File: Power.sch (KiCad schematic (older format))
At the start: 80 parts, among them J3 USB, J4 OTG, Q1 DTA114YKA, SW1 PWRON, SW2 RST, U1 AllWinner-S3(FBGA-234), U3 AXP209(QFN-48), U4 SY8089AAAC, U5 SY6280AAC

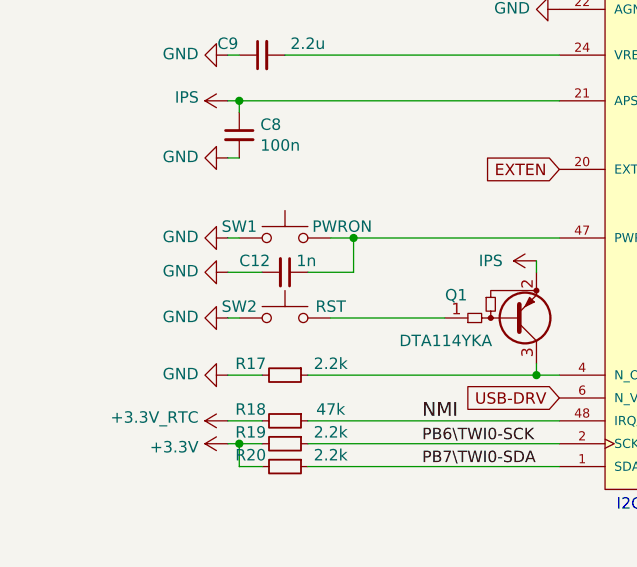
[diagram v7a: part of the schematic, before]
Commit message: update
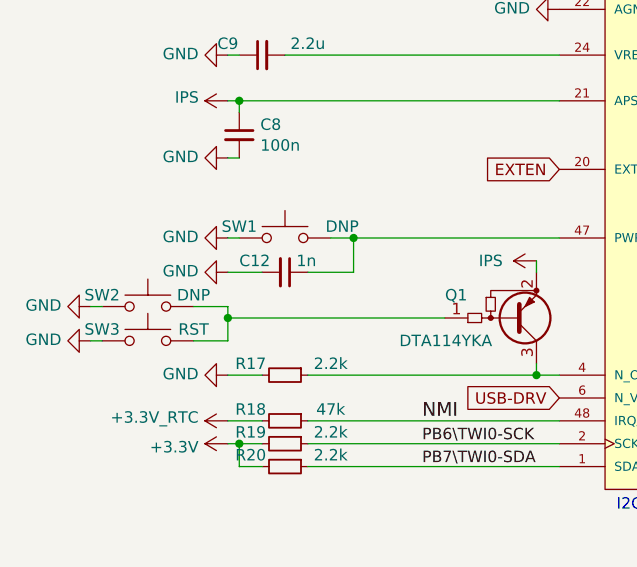
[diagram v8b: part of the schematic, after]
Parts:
- added SW3: RST, otter:SW_SPST_PTS810, symbol Switch:SW_Push
- SW1: value PWRON -> DNP; footprint Button_Switch_SMD:SW_SPST_PTS810 -> otter:SW_SPST_PTS810
- SW2: value RST -> DNP; footprint Button_Switch_SMD:SW_SPST_PTS810 -> otter:SW_SPST_PTS810
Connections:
- net GND: now also SW3.1
- net at Q1.1 (B), SW2.2: now also SW3.2
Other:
- moved on the sheet: SW2
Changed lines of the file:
@@
 L Switch:SW_Push SW2
 U 1 1 6637168B
-P 2050 5300
-F 0 "SW2" H 1850 5350 50  0000 C CNN
-F 1 "RST" H 2250 5350 50  0000 C CNN
-F 2 "Button_Switch_SMD:SW_SPST_PTS810" H 2050 5500 50  0001 C CNN
-F 3 "~" H 2050 5500 50  0001 C CNN
-	1    2050 5300
+P 1450 5250
+F 0 "SW2" H 1250 5300 50  0000 C CNN
+F 1 "DNP" H 1650 5300 50  0000 C CNN
+F 2 "otter:SW_SPST_PTS810" H 1450 5450 50  0001 C CNN
+F 3 "~" H 1450 5450 50  0001 C CNN
+	1    1450 5250
 	1    0    0    -1
 $EndComp
@@
 L S3-OLinuXino_Rev_A:GND #PWR?
 U 1 1 663B8CCA
-P 1800 5300
+P 1200 5250
 AR Path="/5D8A1FAC/663B8CCA" Ref="#PWR?"  Part="1"
 AR Path="/663B8CCA" Ref="#PWR?"  Part="1"
 AR Path="/602ACDF9/663B8CCA" Ref="#PWR0165"  Part="1"
-F 0 "#PWR0165" H 1800 5050 50  0001 C CNN
-F 1 "GND" V 1805 5172 50  0000 R CNN
-F 2 "" H 1800 5300 60  0000 C CNN
-F 3 "" H 1800 5300 60  0000 C CNN
-	1    1800 5300
+F 0 "#PWR0165" H 1200 5000 50  0001 C CNN
+F 1 "GND" V 1205 5122 50  0000 R CNN
+F 2 "" H 1200 5250 60  0000 C CNN
+F 3 "" H 1200 5250 60  0000 C CNN
+	1    1200 5250
 	0    1    -1   0
 $EndComp
 Wire Wire Line
-	1850 5300 1800 5300
+	1250 5250 1200 5250
 $Comp
 L Device:C_Small C?
@@
 P 2050 4950
 F 0 "SW1" H 1850 5000 50  0000 C CNN
-F 1 "PWRON" H 2300 5000 50  0000 C CNN
-F 2 "Button_Switch_SMD:SW_SPST_PTS810" H 2050 5150 50  0001 C CNN
+F 1 "DNP" H 2300 5000 50  0000 C CNN
+F 2 "otter:SW_SPST_PTS810" H 2050 5150 50  0001 C CNN
 F 3 "~" H 2050 5150 50  0001 C CNN
 	1    2050 4950
@@
 $EndComp
 Wire Wire Line
-	2250 5300 2750 5300
-Wire Wire Line
 	2150 5100 2350 5100
 Wire Wire Line
@@
 Wire Wire Line
 	10850 4800 11450 4800
+$Comp
+L Switch:SW_Push SW3
+U 1 1 601100C1
+P 1450 5400
+F 0 "SW3" H 1250 5450 50  0000 C CNN
+F 1 "RST" H 1650 5450 50  0000 C CNN
+F 2 "otter:SW_SPST_PTS810" H 1450 5600 50  0001 C CNN
+F 3 "~" H 1450 5600 50  0001 C CNN
+	1    1450 5400
+	1    0    0    -1
+$EndComp
+$Comp
+L S3-OLinuXino_Rev_A:GND #PWR?
+U 1 1 60166E26
+P 1200 5400
+AR Path="/5D8A1FAC/60166E26" Ref="#PWR?"  Part="1"
+AR Path="/60166E26" Ref="#PWR?"  Part="1"
+AR Path="/602ACDF9/60166E26" Ref="#PWR0134"  Part="1"
+F 0 "#PWR0134" H 1200 5150 50  0001 C CNN
+F 1 "GND" V 1205 5272 50  0000 R CNN
+F 2 "" H 1200 5400 60  0000 C CNN
+F 3 "" H 1200 5400 60  0000 C CNN
+	1    1200 5400
+	0    1    -1   0
+$EndComp
+Wire Wire Line
+	1200 5400 1250 5400
+Wire Wire Line
+	1800 5300 1800 5250
+Wire Wire Line
+	1800 5250 1650 5250
+Wire Wire Line
+	1800 5300 2750 5300
+Wire Wire Line
+	1650 5400 1800 5400
+Wire Wire Line
+	1800 5400 1800 5300
+Connection ~ 1800 5300
 $EndSCHEMATC
